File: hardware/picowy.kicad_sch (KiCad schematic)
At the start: 42 parts, among them J101 Conn_ARM_SWD_TagConnect_TC2030, U101 ER-TP1.44-1, U102 LIS2HH12, U103 FT260Q, U104 ER-OLED1.12-2W, U105 AT24CS04-SSHM, U106 STM32L011G4Ux

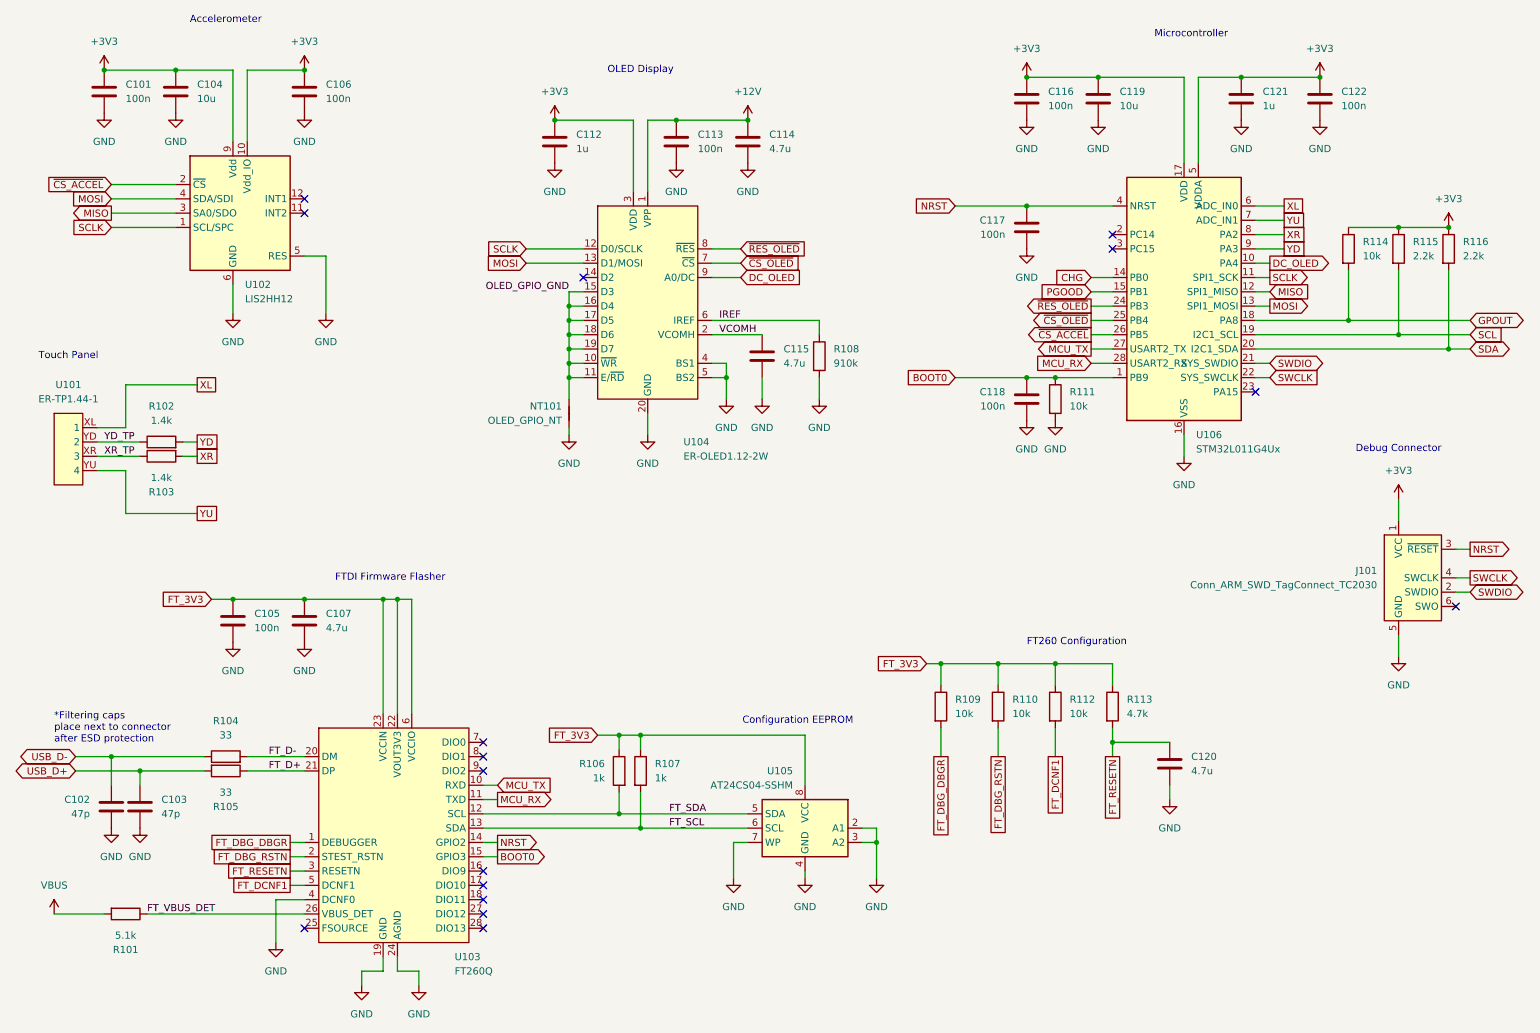
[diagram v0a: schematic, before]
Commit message: Restarting routing
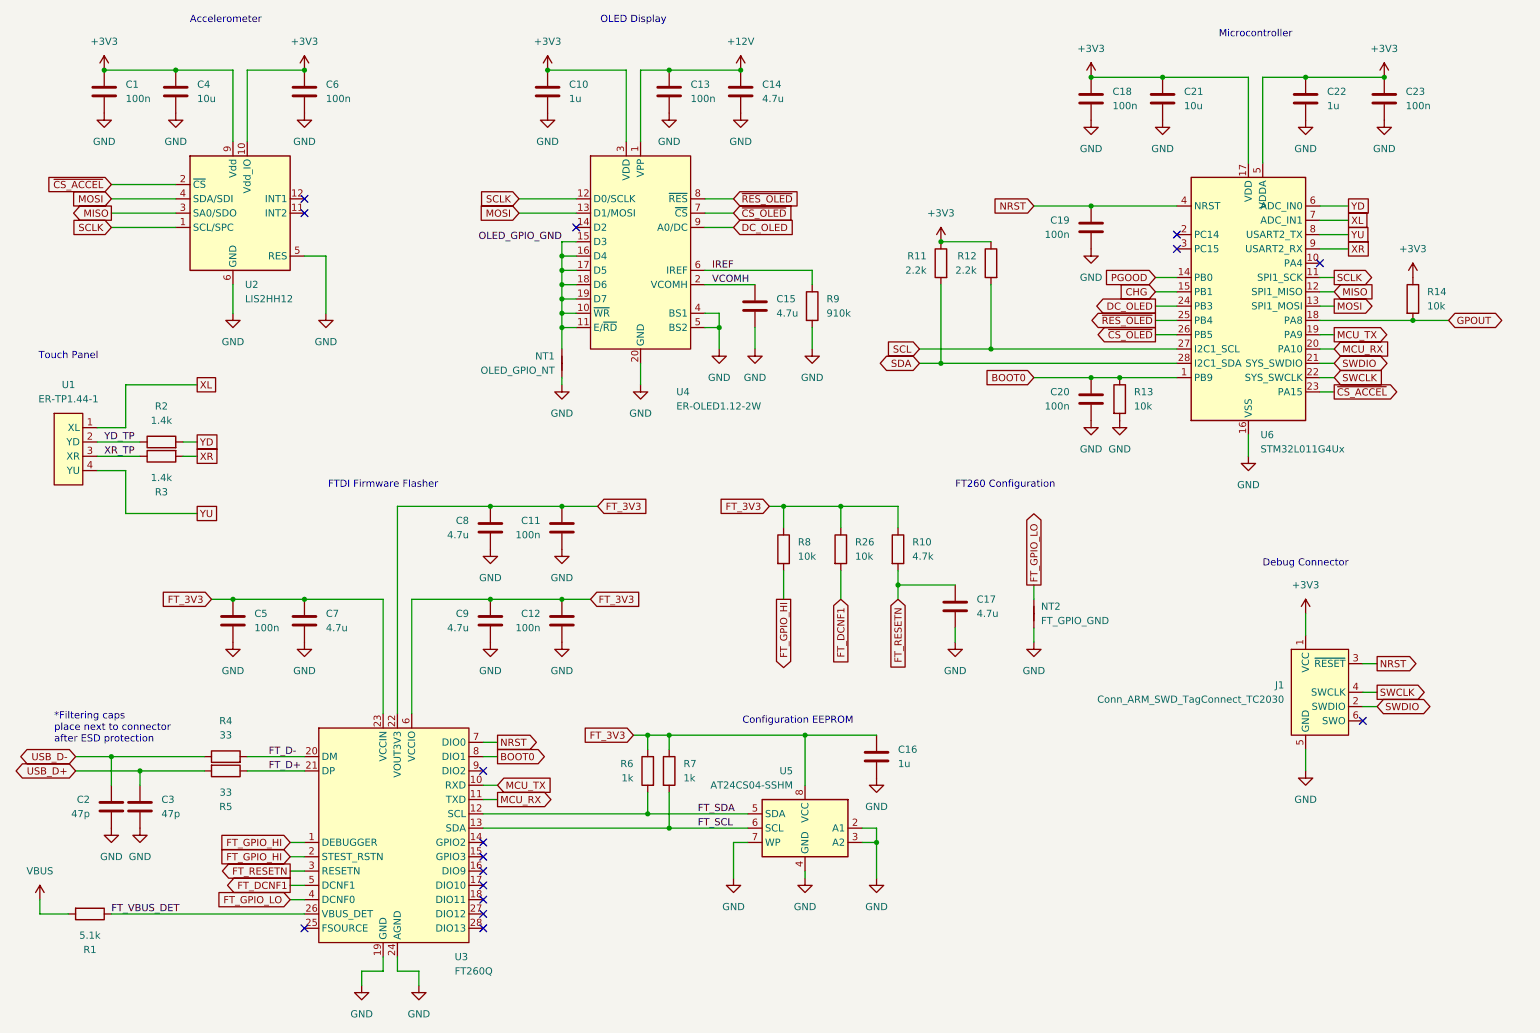
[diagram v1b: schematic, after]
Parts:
- removed R110, R112, R114: 10k, Resistor_SMD:R_0603_1608Metric, symbol Device:R
- removed R115, R116: 2.2k, Resistor_SMD:R_0603_1608Metric, symbol Device:R
- added C11, C12: 100n, Capacitor_SMD:C_0603_1608Metric, symbol Device:C
- added C16: 1u, Capacitor_SMD:C_0603_1608Metric, symbol Device:C
- added C8, C9: 4.7u, Capacitor_SMD:C_0603_1608Metric, symbol Device:C
- added NT2: FT_GPIO_GND, NetTie:NetTie-2_SMD_Pad0.5mm, symbol Device:NetTie_2
- added R11, R12: 2.2k, Resistor_SMD:R_0603_1608Metric, symbol Device:R
- added R14, R26: 10k, Resistor_SMD:R_0603_1608Metric, symbol Device:R
- U3: renamed from U103; footprint Package_DFN_QFN:WQFN-28-1EP_4x4mm_P0.4mm_EP2.7x2.7mm -> picowy_footprints:WQFN-28_FTD; Manufacturer PN FT260Q-T -> FT260S-U
- renumbered C101 to C1, C112 to C10, C113 to C13, C114 to C14, C115 to C15, C120 to C17, C116 to C18, C117 to C19, C102 to C2, C118 to C20, C119 to C21, C121 to C22, C122 to C23, C103 to C3, C104 to C4, C105 to C5, C106 to C6, C107 to C7, J101 to J1, NT101 to NT1, R101 to R1, R113 to R10, R111 to R13, R102 to R2, R103 to R3, R104 to R4, R105 to R5, R106 to R6, R107 to R7, R109 to R8, R108 to R9, U101 to U1, U102 to U2, U104 to U4, U105 to U5, U106 to U6
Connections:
- net FT_DBG_RSTN is gone; now on net FT_GPIO_HI: U3.2 (STEST_RSTN)
- net +3V3: now also R11.1, R12.1, R14.1
- net BOOT0: now also U3.8 (DIO1); no longer U3.15 (DIO8)
- net CHG: now also U6.15 (PB1); no longer U6.14 (PB0)
- net DC_OLED: now also U6.24 (PB3); no longer U6.10 (PA4)
- net FT_3V3: now also C11.1, C12.1, C16.1, C8.1, C9.1, R26.1
- net FT_DCNF1: now also R26.2
- net GND: now also C11.2, C12.2, C16.2, C8.2, C9.2, NT2.1; no longer U3.4 (DCNF0)
- net GPOUT: now also R14.2
- net MCU_RX: now also U6.20 (PA10); no longer U6.28 (PB7)
- net MCU_TX: now also U6.19 (PA9); no longer U6.27 (PB6)
- net NRST: now also U3.7 (DIO0); no longer U3.14 (DIO7)
- net PGOOD: now also U6.14 (PB0); no longer U6.15 (PB1)
- net SCL: now also U6.27 (PB6), R12.2; no longer U6.19 (PA9)
- net SDA: now also U6.28 (PB7), R11.2; no longer U6.20 (PA10)
- net XL: now also U1.1 (XL), U6.7 (PA1); no longer U1.XL (1), U6.6 (PA0)
- net XR: now also U6.9 (PA3); no longer U6.8 (PA2)
- net XR_TP: now also U1.3 (XR); no longer U1.XR (3)
- net YD: now also U6.6 (PA0); no longer U6.9 (PA3)
- net YD_TP: now also U1.2 (YD); no longer U1.YD (2)
- net YU: now also U1.4 (YU), U6.8 (PA2); no longer U1.YU (4), U6.7 (PA1)
- net ~{CS_ACCEL}: now also U6.23 (PA15); no longer U6.26 (PB5)
- net ~{CS_OLED}: now also U6.26 (PB5); no longer U6.25 (PB4)
- net ~{RES_OLED}: now also U6.25 (PB4); no longer U6.24 (PB3)
- net FT_DBG_DBGR renamed FT_GPIO_HI
- new net FT_GPIO_LO: NT2.2, U3.4 (DCNF0)
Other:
- moved on the sheet: C10, C13, C14, C15, C17, C18, C19, C20, C21, C22, C23, J1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
